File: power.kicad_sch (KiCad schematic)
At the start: 128 parts, among them Q2 BC817-25W, Q3 DZDH0401DW, Q4 DZDH0401DW, Q5 SI7613DN-T1-GE3, Q6 SI7613DN-T1-GE3, U1 LT8350RV, U2 MP2386GG, U3 TPS65983BAZBHR

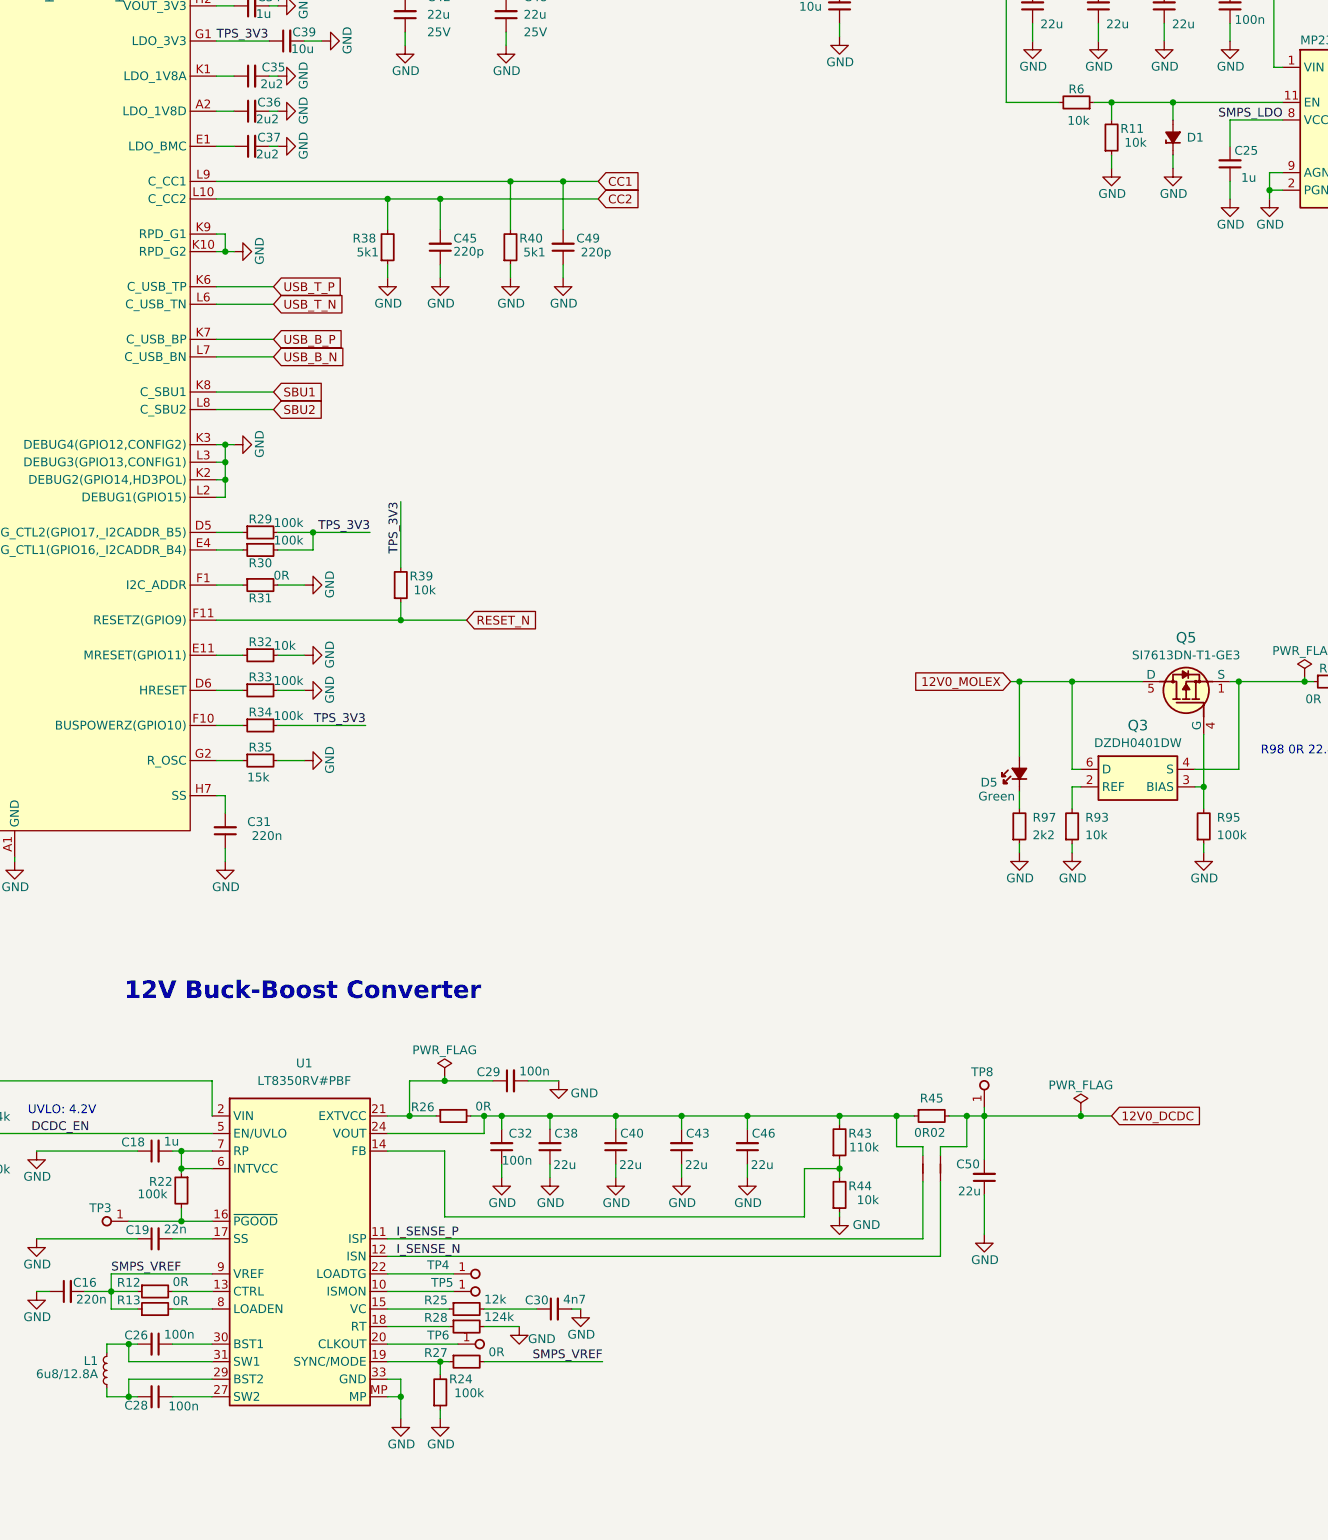
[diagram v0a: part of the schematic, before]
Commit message: [#58582] Clean DRC
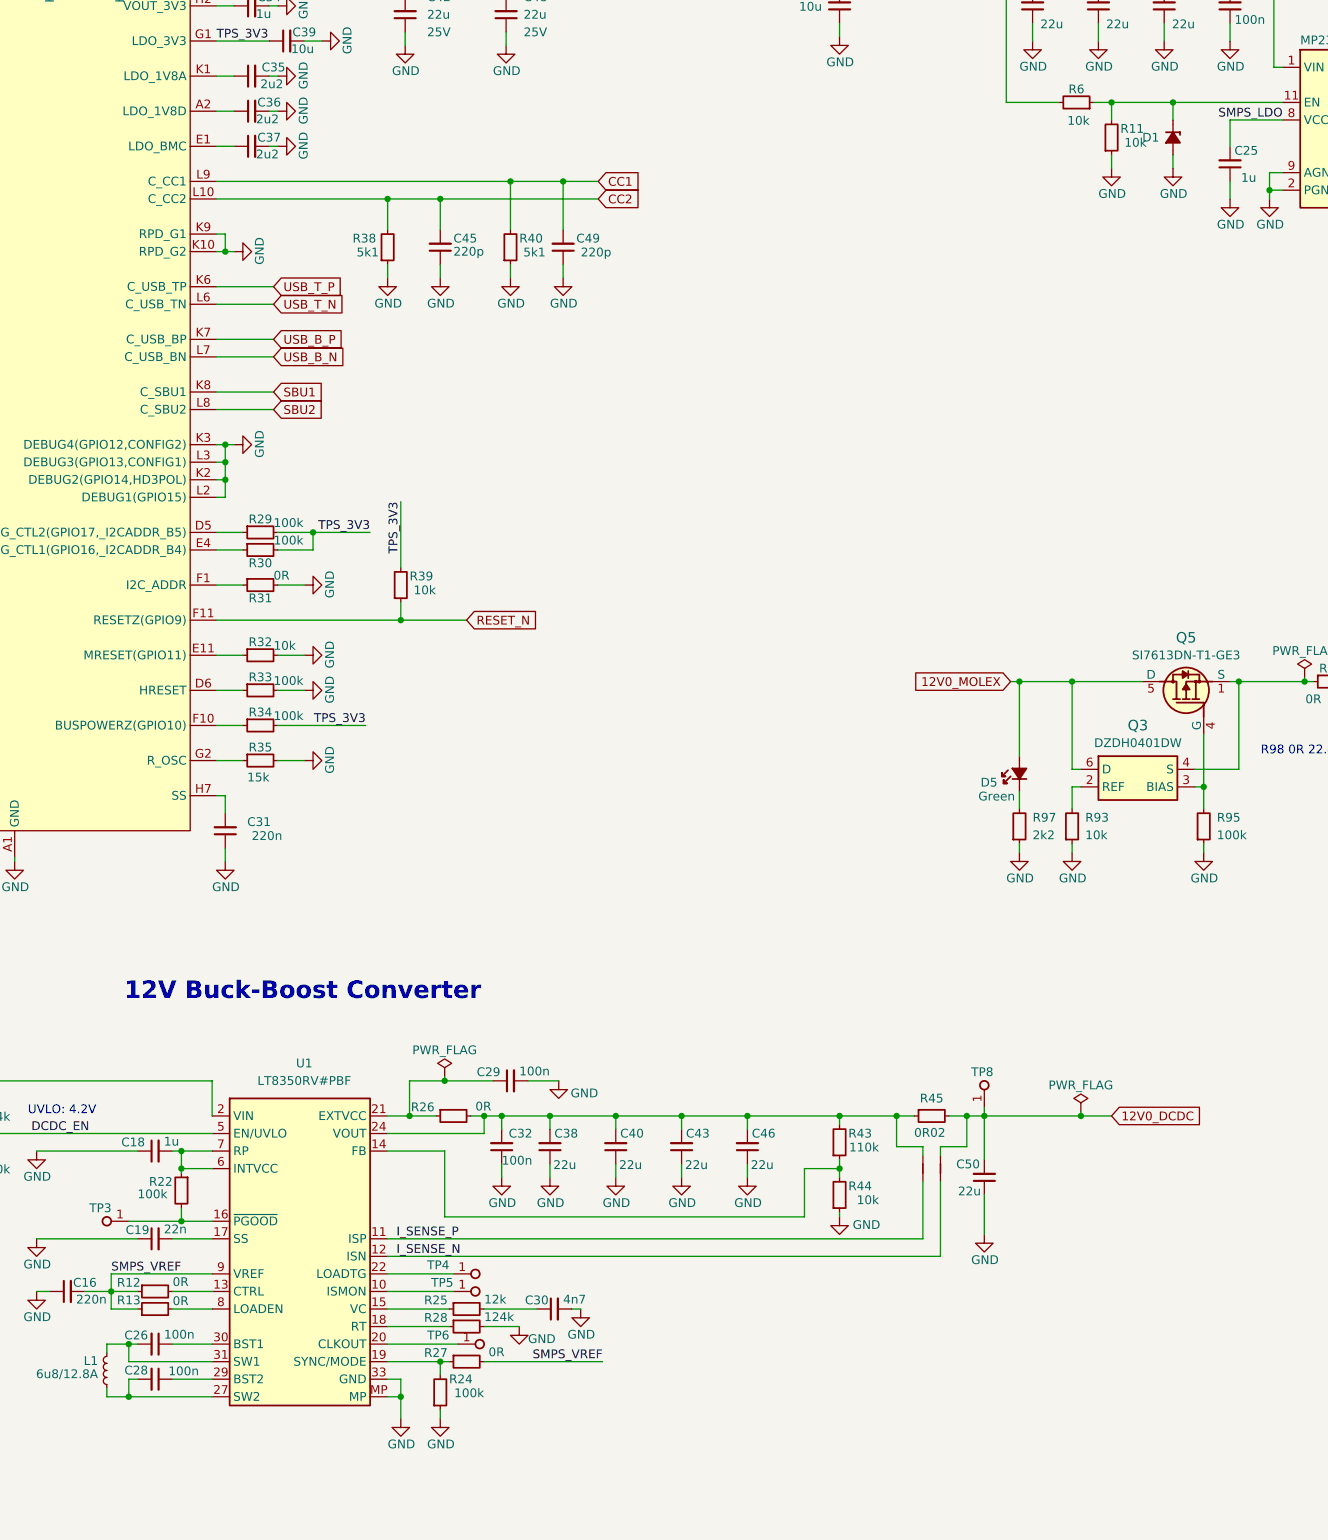
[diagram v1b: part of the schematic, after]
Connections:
- net GND: now also D1.2 (A); no longer D1.1 (C)
- net at R11.2, R6.1, U2.11 (EN): now also D1.1 (C); no longer D1.2 (A)
- net at U1.27 (SW2), U1.28 (SW2): now also C28.2, L1.2; no longer C28.1
- new net: C28.1, U1.29 (BST2)
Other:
- moved on the sheet: C28, D1
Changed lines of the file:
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@@
   (junction (at 135.89 116.84) (diameter 0) (color 0 0 0 0)
   )
-  (junction (at 161.29 249.555) (diameter 0) (color 0 0 0 0)
-  )
   (junction (at 329.565 67.31) (diameter 0) (color 0 0 0 0)
   )
@@
   (junction (at 161.925 43.18) (diameter 0) (color 0 0 0 0)
   )
-  (junction (at 121.92 249.555) (diameter 0) (color 0 0 0 0)
-  )
   (junction (at 258.445 146.05) (diameter 0) (color 0 0 0 0)
   )
@@
   (junction (at 99.695 203.835) (diameter 0) (color 0 0 0 0)
   )
+  (junction (at 161.29 249.555) (diameter 0) (color 0 0 0 0)
+  )
   (junction (at 74.93 58.42) (diameter 0) (color 0 0 0 0)
   )
@@
   (junction (at 224.79 216.535) (diameter 0) (color 0 0 0 0)
   )
+  (junction (at 121.92 249.555) (diameter 0) (color 0 0 0 0)
+  )
   (junction (at 30.48 57.15) (diameter 0) (color 0 0 0 0)
   )
@@
     (stroke (width 0) (type default))
   )
+  (wire (pts (xy 121.92 247.015) (xy 121.92 249.555))
+    (stroke (width 0) (type default))
+  )
   (wire (pts (xy 57.15 242.57) (xy 60.325 242.57))
     (stroke (width 0) (type default))
@@
     (stroke (width 0) (type default))
   )
+  (wire (pts (xy 121.92 249.555) (xy 133.985 249.555))
+    (stroke (width 0) (type default))
+  )
   (wire (pts (xy 176.53 43.18) (xy 176.53 46.99))
     (stroke (width 0) (type default))
@@
     (stroke (width 0) (type default))
   )
-  (wire (pts (xy 128.27 249.555) (xy 133.985 249.555))
+  (wire (pts (xy 128.27 247.015) (xy 133.985 247.015))
     (stroke (width 0) (type default))
   )
@@
     (stroke (width 0) (type default))
   )
-  (wire (pts (xy 121.92 247.015) (xy 133.985 247.015))
-    (stroke (width 0) (type default))
-  )
   (wire (pts (xy 121.92 224.155) (xy 129.54 224.155))
     (stroke (width 0) (type default))
@@
     (stroke (width 0) (type default))
   )
-  (wire (pts (xy 121.92 249.555) (xy 123.19 249.555))
+  (wire (pts (xy 121.92 247.015) (xy 123.19 247.015))
     (stroke (width 0) (type default))
   )
@@
     (stroke (width 0) (type default))
   )
+  (wire (pts (xy 159.385 249.555) (xy 161.29 249.555))
+    (stroke (width 0) (type default))
+  )
   (wire (pts (xy 67.31 48.26) (xy 74.93 48.26))
     (stroke (width 0) (type default))
@@
     (stroke (width 0) (type default))
   )
-  (wire (pts (xy 121.92 247.015) (xy 121.92 249.555))
-    (stroke (width 0) (type default))
-  )
   (wire (pts (xy 245.745 207.645) (xy 245.745 208.915))
     (stroke (width 0) (type default))
@@
     (stroke (width 0) (type default))
   )
-  (wire (pts (xy 159.385 249.555) (xy 161.29 249.555))
-    (stroke (width 0) (type default))
-  )
   (wire (pts (xy 159.385 229.235) (xy 239.395 229.235))
     (stroke (width 0) (type default))
@@
     (stroke (width 0) (type default))
   )
+  (wire (pts (xy 161.29 249.555) (xy 161.29 252.73))
+    (stroke (width 0) (type default))
+  )
   (wire (pts (xy 69.85 203.835) (xy 69.85 205.74))
     (stroke (width 0) (type default))
@@
     (stroke (width 0) (type default))
   )
-  (wire (pts (xy 161.29 249.555) (xy 161.29 252.73))
-    (stroke (width 0) (type default))
-  )
   (wire (pts (xy 121.92 244.475) (xy 133.985 244.475))
     (stroke (width 0) (type default))
@@
     )
   )
-  (symbol (lib_id "antmicroDiodesZenerSingle:MM3Z3V3C") (at 273.05 69.85 90) (unit 1)
+  (symbol (lib_id "antmicroDiodesZenerSingle:MM3Z3V3C") (at 273.05 64.77 270) (unit 1)
     (in_bom yes) (on_board yes) (dnp no)
-    (property "Reference" "D1" (at 277.495 67.31 90)
+    (property "Reference" "D1" (at 268.605 67.31 90)
       (effects (font (size 1.27 1.27) (thickness 0.15)) (justify left))
     )
-    (property "Value" "MM3Z3V3C" (at 288.29 46.99 0)
+    (property "Value" "MM3Z3V3C" (at 257.81 87.63 0)
       (effects (font (size 1.27 1.27) (thickness 0.15)) (justify left bottom) hide)
     )
-    (property "Footprint" "antmicro-footprints:D_SOD-323F" (at 283.21 46.99 0)
+    (property "Footprint" "antmicro-footprints:D_SOD-323F" (at 262.89 87.63 0)
       (effects (font (size 1.27 1.27) (thickness 0.15)) (justify left bottom) hide)
     )
-    (property "Datasheet" "https://www.onsemi.com/download/data-sheet/pdf/mm3z9v1c-d.pdf" (at 285.75 46.99 0)
+    (property "Datasheet" "https://www.onsemi.com/download/data-sheet/pdf/mm3z9v1c-d.pdf" (at 260.35 87.63 0)
       (effects (font (size 1.27 1.27) (thickness 0.15)) (justify left bottom) hide)
     )
-    (property "MPN" "MM3Z3V3C" (at 277.495 52.07 90)
+    (property "MPN" "MM3Z3V3C" (at 268.605 82.55 90)
       (effects (font (size 1.27 1.27) (thickness 0.15)) (justify left bottom) hide)
     )
-    (property "Manufacturer" "ON Semiconductor" (at 290.83 46.99 0)
+    (property "Manufacturer" "ON Semiconductor" (at 255.27 87.63 0)
       (effects (font (size 1.27 1.27) (thickness 0.15)) (justify left bottom) hide)
     )
-    (property "License" "Apache-2.0" (at 295.91 46.99 0)
+    (property "License" "Apache-2.0" (at 250.19 87.63 0)
       (effects (font (size 1.27 1.27) (thickness 0.15)) (justify left bottom) hide)
     )
-    (property "Author" "Antmicro" (at 293.37 46.99 0)
+    (property "Author" "Antmicro" (at 252.73 87.63 0)
       (effects (font (size 1.27 1.27) (thickness 0.15)) (justify left bottom) hide)
     )
@@
     )
   )
-  (symbol (lib_id "antmicroCapacitors0402:C_100n_0402") (at 128.27 249.555 180) (unit 1)
+  (symbol (lib_id "antmicroCapacitors0402:C_100n_0402") (at 128.27 247.015 180) (unit 1)
     (in_bom yes) (on_board yes) (dnp no)
-    (property "Reference" "C28" (at 121.285 250.825 0)
+    (property "Reference" "C28" (at 121.285 245.745 0)
       (effects (font (size 1.27 1.27) (thickness 0.15)) (justify right))
     )
-    (property "Value" "C_100n_0402" (at 107.95 239.395 0)
+    (property "Value" "C_100n_0402" (at 107.95 236.855 0)
       (effects (font (size 1.27 1.27) (thickness 0.15)) (justify left bottom) hide)
     )
-    (property "Footprint" "antmicro-footprints:C_0402_1005Metric" (at 107.95 236.855 0)
+    (property "Footprint" "antmicro-footprints:C_0402_1005Metric" (at 107.95 234.315 0)
       (effects (font (size 1.27 1.27) (thickness 0.15)) (justify left bottom) hide)
     )
-    (property "Datasheet" "https://www.murata.com/products/productdetail?partno=GRM155R61H104KE14%23" (at 107.95 234.315 0)
+    (property "Datasheet" "https://www.murata.com/products/productdetail?partno=GRM155R61H104KE14%23" (at 107.95 231.775 0)
       (effects (font (size 1.27 1.27) (thickness 0.15)) (justify left bottom) hide)
     )
-    (property "MPN" "GRM155R61H104KE14D" (at 107.95 231.775 0)
+    (property "MPN" "GRM155R61H104KE14D" (at 107.95 229.235 0)
       (effects (font (size 1.27 1.27) (thickness 0.15)) (justify left bottom) hide)
     )
-    (property "Manufacturer" "Murata" (at 107.95 229.235 0)
+    (property "Manufacturer" "Murata" (at 107.95 226.695 0)
       (effects (font (size 1.27 1.27) (thickness 0.15)) (justify left bottom) hide)
     )
-    (property "License" "Apache-2.0" (at 107.95 226.695 0)
+    (property "License" "Apache-2.0" (at 107.95 224.155 0)
       (effects (font (size 1.27 1.27) (thickness 0.15)) (justify left bottom) hide)
     )
-    (property "Val" "100n" (at 132.08 250.19 0)
+    (property "Val" "100n" (at 132.08 245.11 0)
       (effects (font (size 1.27 1.27) (thickness 0.15)) (justify left bottom))
     )
-    (property "Voltage" "50V" (at 107.95 221.615 0)
+    (property "Voltage" "50V" (at 107.95 219.075 0)
       (effects (font (size 1.27 1.27)) (justify left bottom) hide)
     )
-    (property "Dielectric" "X5R" (at 107.95 219.075 0)
+    (property "Dielectric" "X5R" (at 107.95 216.535 0)
       (effects (font (size 1.27 1.27)) (justify left bottom) hide)
     )
-    (property "Author" "Antmicro" (at 107.95 224.155 0)
+    (property "Author" "Antmicro" (at 107.95 221.615 0)
       (effects (font (size 1.27 1.27) (thickness 0.15)) (justify left bottom) hide)
     )
